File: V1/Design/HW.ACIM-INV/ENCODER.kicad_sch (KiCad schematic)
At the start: 22 parts, among them J10 ENCODER PORT, J11 ENCODER, Q4 60V/265mA, Q5 60V/265mA, Q6 60V/265mA, Q7 60V/265mA

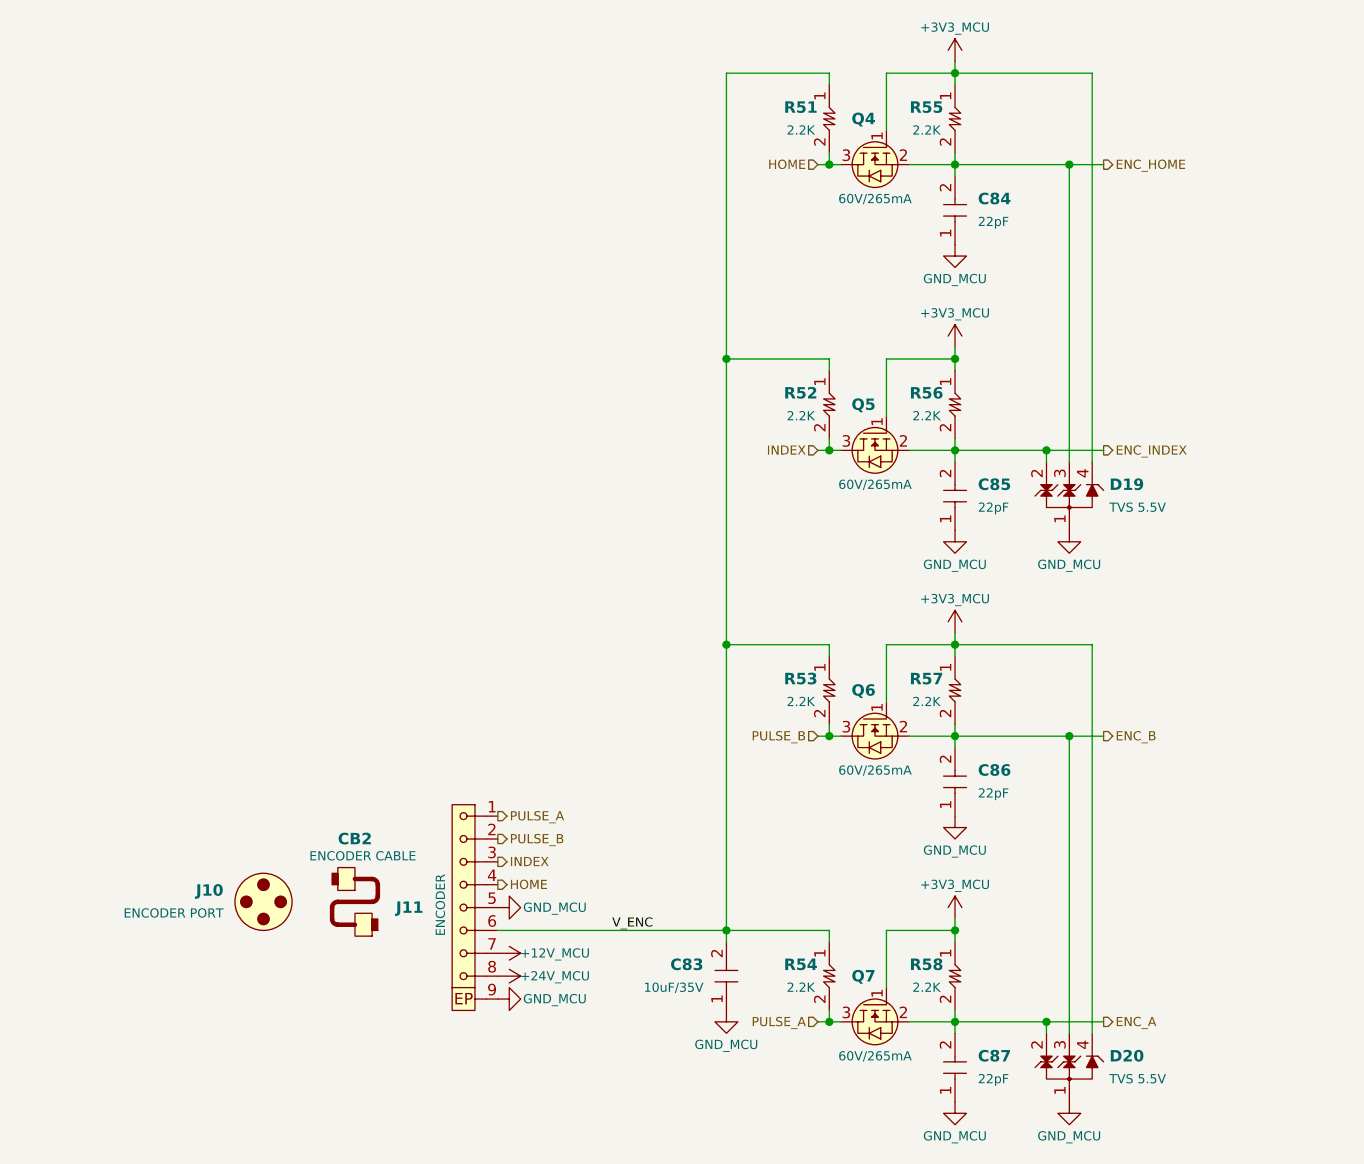
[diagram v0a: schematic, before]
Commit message: V1 schematic update 18
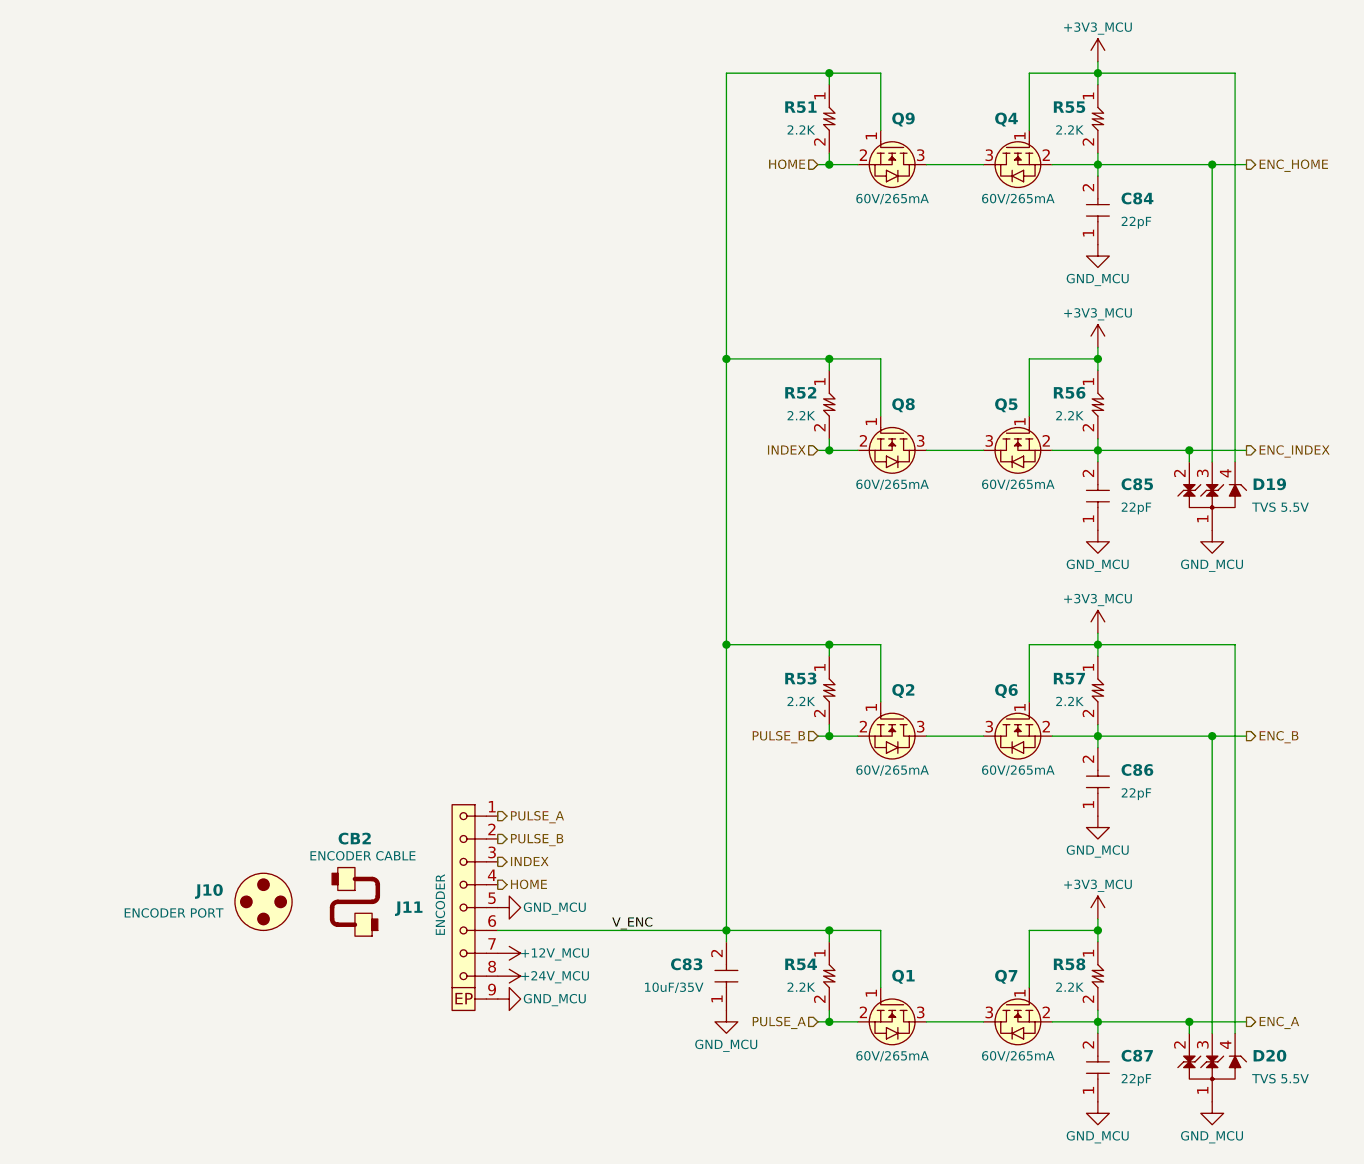
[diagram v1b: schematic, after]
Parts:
- added Q1, Q2, Q8, Q9: 60V/265mA, SAMPI:SOT23, symbol SAMPI:FET_N-CH
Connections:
- net HOME: now also Q9.2 (S); no longer Q4.3 (D)
- net INDEX: now also Q8.2 (S); no longer Q5.3 (D)
- net PULSE_A: now also Q1.2 (S); no longer Q7.3 (D)
- net PULSE_B: now also Q2.2 (S); no longer Q6.3 (D)
- net V_ENC: now also Q1.1 (G), Q2.1 (G), Q8.1 (G), Q9.1 (G)
- new net: Q4.3 (D), Q9.3 (D)
- new net: Q1.3 (D), Q7.3 (D)
- new net: Q2.3 (D), Q6.3 (D)
- new net: Q5.3 (D), Q8.3 (D)
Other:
- moved on the sheet: C84, C85, C86, C87, D19, D20, Q4, Q5, Q6, Q7, R55, R56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

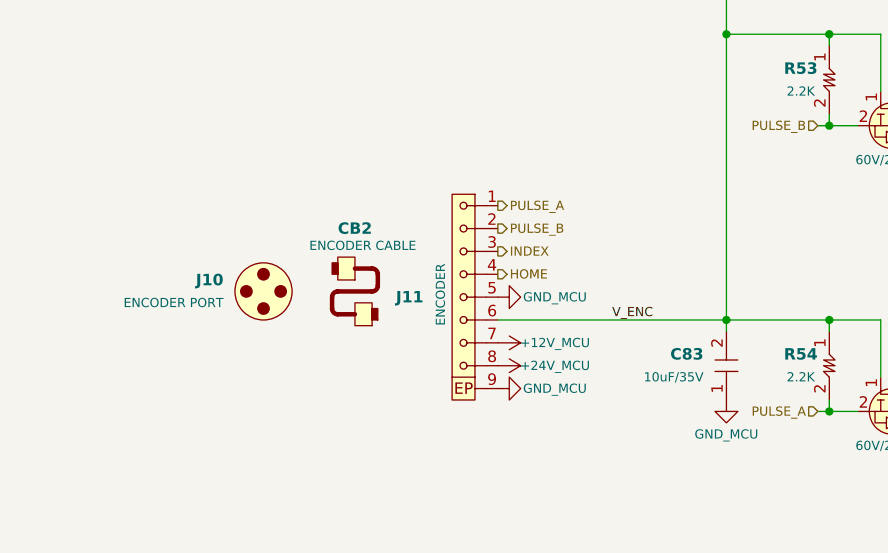
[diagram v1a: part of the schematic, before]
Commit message: V1 schematic update 20
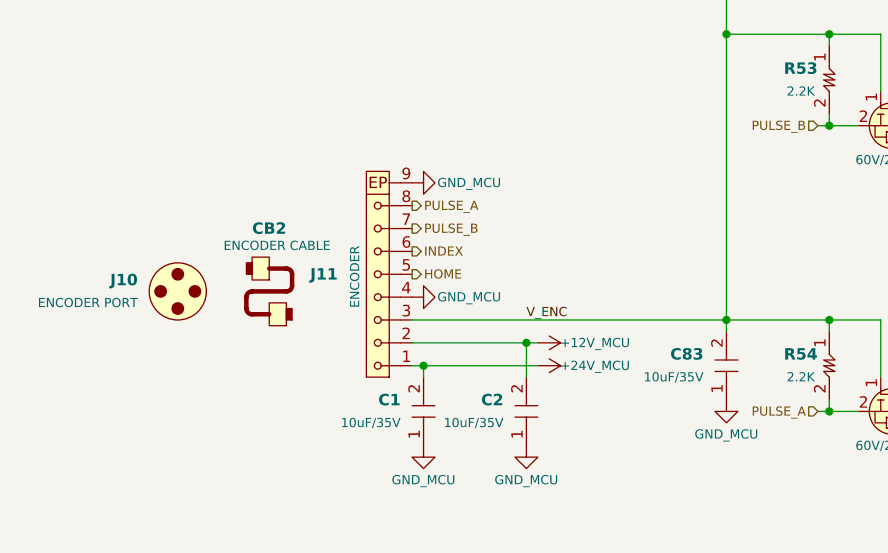
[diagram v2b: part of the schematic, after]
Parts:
- added C1, C2: 10uF/35V, SAMPI:CAP1206, symbol SAMPI:CERCAP
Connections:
- net +12V_MCU: now also J11.2, C2.2; no longer J11.7
- net +24V_MCU: now also J11.1, C1.2; no longer J11.8
- net GND_MCU: now also J11.4, C1.1, C2.1; no longer J11.5
- net HOME: now also J11.5; no longer J11.4
- net INDEX: now also J11.6; no longer J11.3
- net PULSE_A: now also J11.8; no longer J11.1
- net PULSE_B: now also J11.7; no longer J11.2
- net V_ENC: now also J11.3; no longer J11.6
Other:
- moved on the sheet: CB2, J10, J11
